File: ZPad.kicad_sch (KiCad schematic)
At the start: 0 parts

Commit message: Schematic done
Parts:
- added D1, D2, D3, D4, D5, D6, D7, D8: 1N4148, Diode_THT:D_DO-35_SOD27_P7.62mm_Horizontal, symbol Diode:1N4148
- added SW1, SW2, SW3, SW4, SW5, SW6, SW7, SW8: SW_Push, symbol Switch:SW_Push
- added SW10: RotaryEncoder, symbol Device:RotaryEncoder
- added SW9: RotaryEncoder_Switch, symbol Device:RotaryEncoder_Switch
- added U1: MOUDLE-SEEEDUINO-XIAO, symbol XIAO_RP2040:MOUDLE-SEEEDUINO-XIAO
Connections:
- new net: D6.2 (A), SW6.1
- new net: D1.2 (A), SW1.1
- new net: D5.2 (A), SW5.1
- new net: D7.2 (A), SW7.1
- new net: D4.2 (A), SW4.1
- new net: D2.2 (A), SW2.1
- new net: D8.2 (A), SW8.1
- new net: D3.2 (A), SW3.1
- new net +3V3: U1.12 (3V3)
- new net +5V: U1.14 (5V)
- new net COL0: SW1.2, SW5.2, U1.1 (PA02_A0_D0)
- new net COL1: SW2.2, SW6.2, U1.2 (PA4_A1_D1)
- new net COL2: SW3.2, SW7.2, U1.3 (PA10_A2_D2)
- new net COL3: SW4.2, SW8.2, U1.4 (PA11_A3_D3)
- new net GND: SW10.C, SW9.C, SW9.S2, U1.13 (GND)
- new net ROW0: D1.1 (K), D2.1 (K), D3.1 (K), D4.1 (K), U1.11 (PA6_A10_D10_MOSI)
- new net ROW1: D5.1 (K), D6.1 (K), D7.1 (K), D8.1 (K), U1.10 (PA5_A9_D9_MISO)
- new net Rotary_A: SW10.A, U1.9 (PA7_A8_D8_SCK)
- new net Rotary_B: SW10.B, U1.8 (PB09_A7_D7_RX)
- new net Rotary_Sw_A: SW9.A, U1.5 (PA8_A4_D4_SDA)
- new net Rotary_Sw_B: SW9.B, U1.6 (PA9_A5_D5_SCL)
- new net Rotary_Sw_S1: SW9.S1, U1.7 (PB08_A6_D6_TX)
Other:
- note added: "Matrix wiring"
- note added: "RP2040"
- note added: "Rotary Encoder"
- note added: "Rotary Encoder (with Switch)"

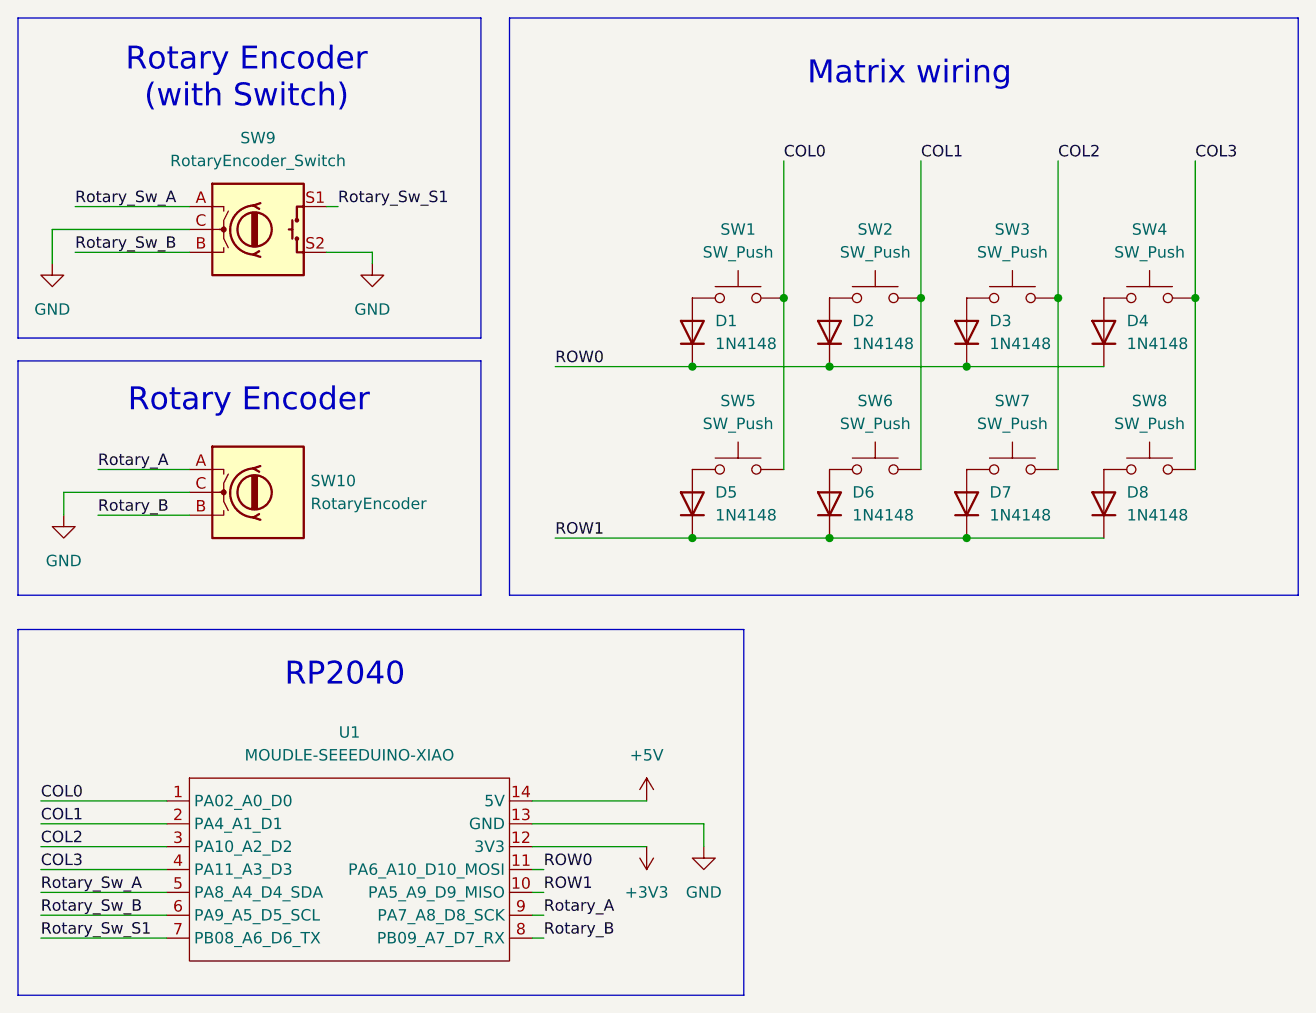
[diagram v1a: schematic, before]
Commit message: Finally the schematic is actually done
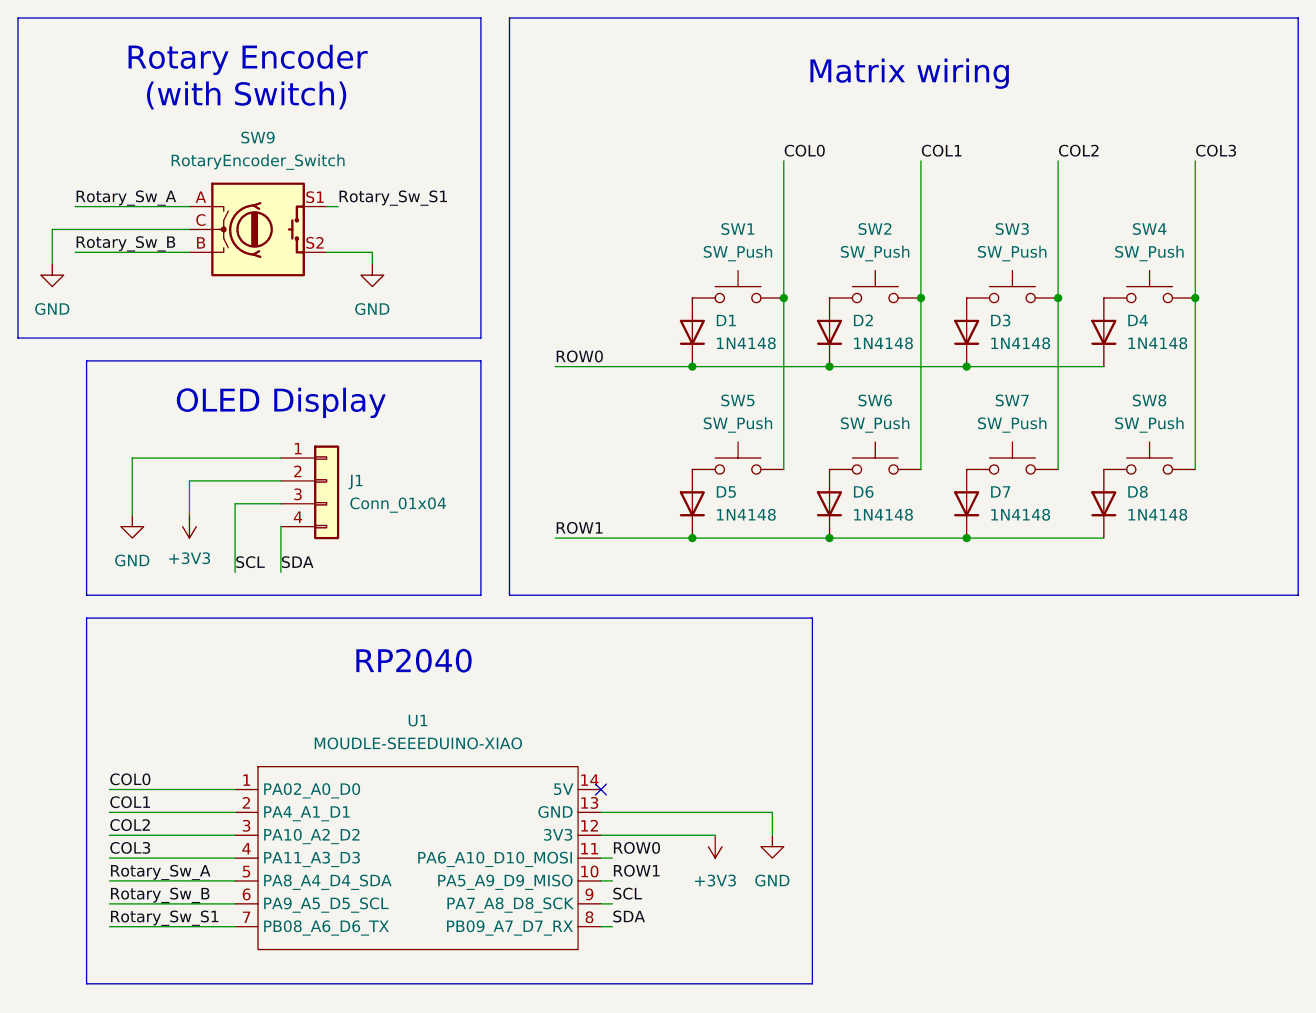
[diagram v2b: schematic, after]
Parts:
- removed SW10: RotaryEncoder, symbol Device:RotaryEncoder
- added J1: Conn_01x04, KiCad-SSD1306-0.91-OLED-4pin-128x32:SSD1306-0.91-OLED-4pin-128x32, symbol Connector_Generic:Conn_01x04
- SW1, SW2, SW3, SW4, SW5, SW6, SW7, SW8: footprint (none) -> Button_Switch_Keyboard:SW_Cherry_MX_1.00u_PCB
- SW9: footprint (none) -> Rotary_Encoder:RotaryEncoder_Alps_EC11E-Switch_Vertical_H20mm
- U1: footprint (none) -> footprints:XIAO-Generic-Hybrid-14P-2.54-21X17.8MM
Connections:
- net +3V3: now also J1.2 (Pin_2)
- net GND: now also J1.1 (Pin_1)
- net +5V: no longer names the net of U1.14 (5V)
- net Rotary_A renamed SCL
- net SCL: now also J1.3 (Pin_3)
- net Rotary_B renamed SDA
- net SDA: now also J1.4 (Pin_4)
- no-connect marks 0 -> 1
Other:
- note added: "OLED Display"
- note removed: "Rotary Encoder"
- moved on the sheet: U1
